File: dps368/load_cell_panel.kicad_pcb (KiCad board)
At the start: 2 copper layers, 50 x 46 mm, 96 parts, among them J1 Conn_01x05_Female, U1 DPS368XTSA1

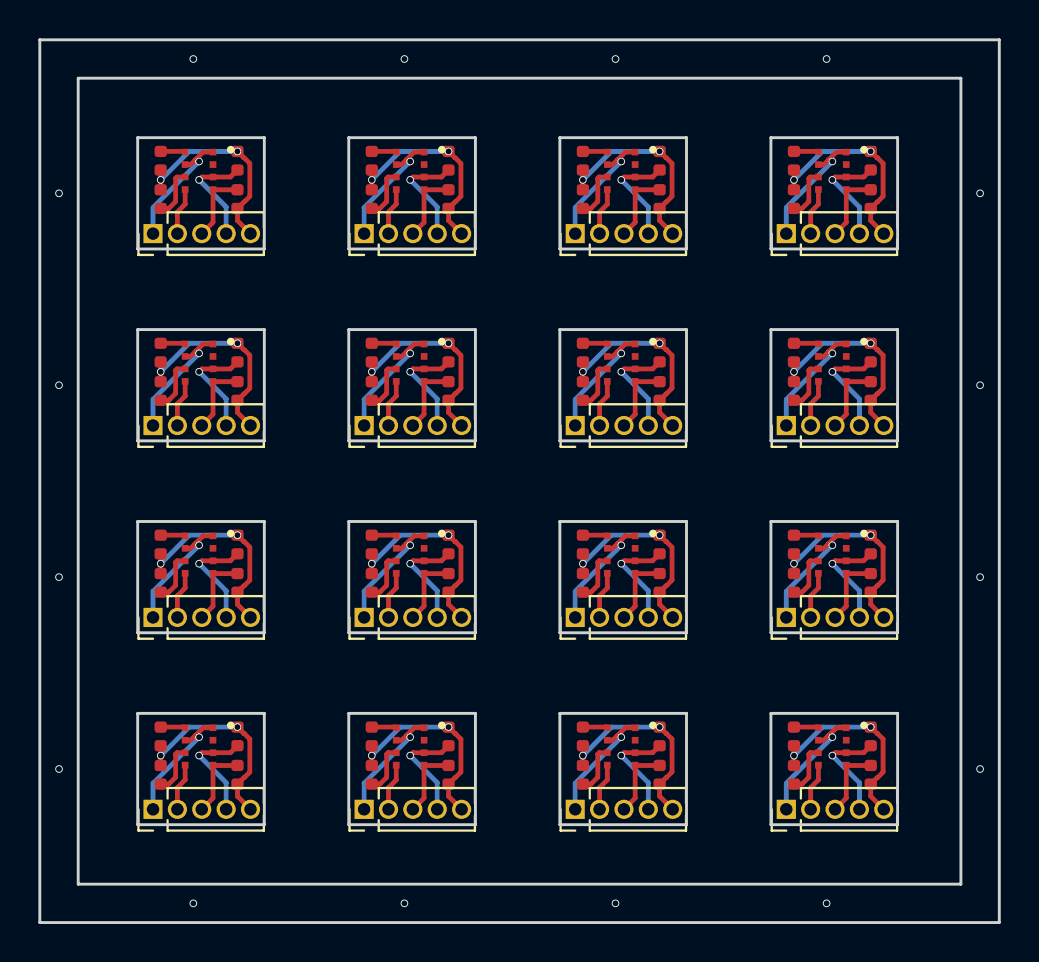
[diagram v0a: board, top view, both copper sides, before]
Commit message: goddamn it
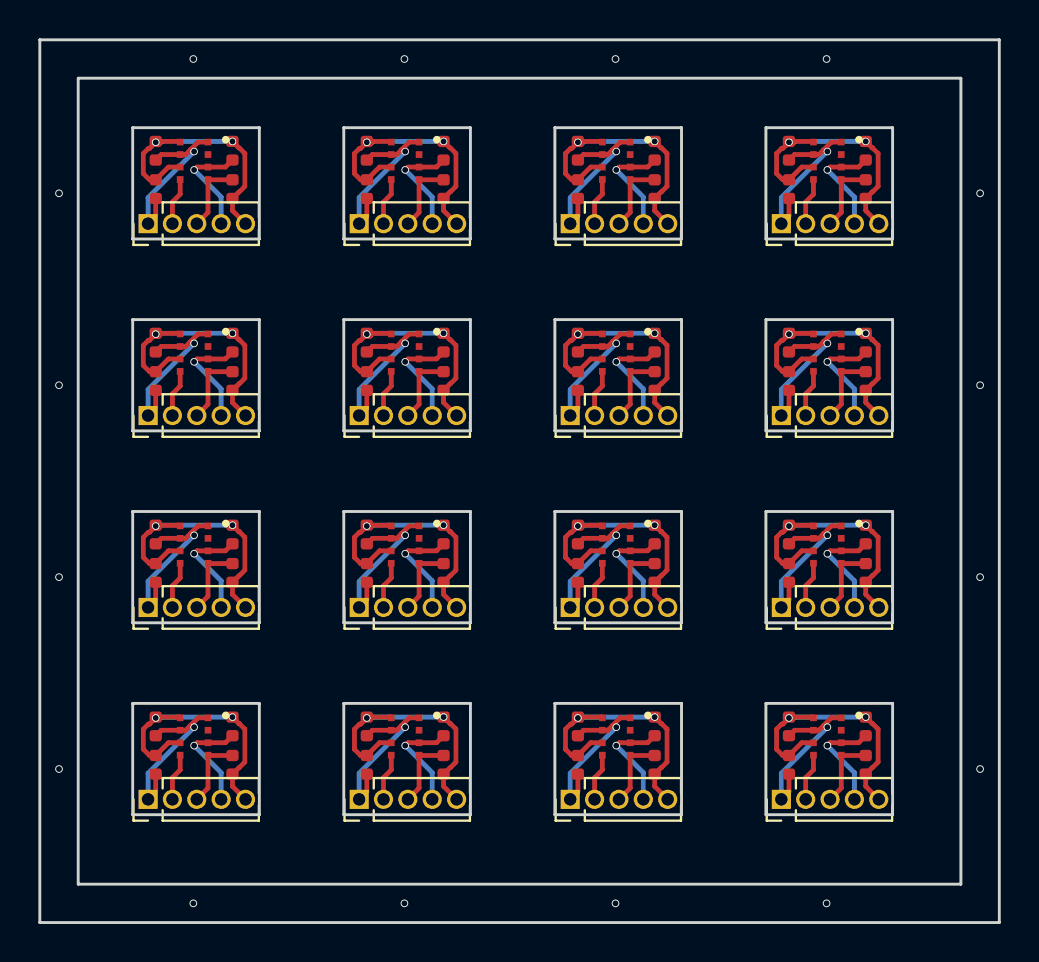
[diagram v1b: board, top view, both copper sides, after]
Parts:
- removed the C1 at (164.3, 101.3)
- removed the C1 at (153.3, 81.3)
- removed the C1 at (142.3, 81.3)
- removed the C1 at (131.3, 81.3)
- removed the C1 at (164.3, 71.3)
- removed the C1 at (153.3, 71.3)
- removed the C1 at (142.3, 71.3)
- removed the C1 at (153.3, 101.3)
- removed the C1 at (142.3, 101.3)
- removed the C1 at (131.3, 101.3)
- removed the C1 at (164.3, 91.3)
- removed the C1 at (153.3, 91.3)
- removed the C1 at (142.3, 91.3)
- removed the C1 at (131.3, 91.3)
- removed the C1 at (164.3, 81.3)
- removed the C2 at (164.3, 103.3)
- removed the C2 at (153.3, 83.3)
- removed the C2 at (142.3, 83.3)
- removed the C2 at (131.3, 83.3)
- removed the C2 at (164.3, 73.3)
- removed the C2 at (153.3, 73.3)
- removed the C2 at (142.3, 73.3)
- removed the C2 at (153.3, 103.3)
- removed the C2 at (142.3, 103.3)
- removed the C2 at (131.3, 103.3)
- removed the C2 at (164.3, 93.3)
- removed the C2 at (153.3, 93.3)
- removed the C2 at (142.3, 93.3)
- removed the C2 at (131.3, 93.3)
- removed the C2 at (164.3, 83.3)
- removed the J1 at (163.9, 105.1)
- removed the J1 at (152.9, 85.1)
- removed the J1 at (141.9, 85.1)
- removed the J1 at (130.9, 85.1)
- removed the J1 at (163.9, 75.1)
- removed the J1 at (152.9, 75.1)
- removed the J1 at (141.9, 75.1)
- removed the J1 at (152.9, 105.1)
- removed the J1 at (141.9, 105.1)
- removed the J1 at (130.9, 105.1)
- removed the J1 at (163.9, 95.1)
- removed the J1 at (152.9, 95.1)
- removed the J1 at (141.9, 95.1)
- removed the J1 at (130.9, 95.1)
- removed the J1 at (163.9, 85.1)
- removed the R1 at (168.3, 103.3)
- removed the R1 at (157.3, 83.3)
- removed the R1 at (146.3, 83.3)
- removed the R1 at (135.3, 83.3)
- removed the R1 at (168.3, 73.3)
- removed the R1 at (157.3, 73.3)
- removed the R1 at (146.3, 73.3)
- removed the R1 at (157.3, 103.3)
- removed the R1 at (146.3, 103.3)
- removed the R1 at (135.3, 103.3)
- removed the R1 at (168.3, 93.3)
- removed the R1 at (157.3, 93.3)
- removed the R1 at (146.3, 93.3)
- removed the R1 at (135.3, 93.3)
- removed the R1 at (168.3, 83.3)
- removed the R2 at (168.3, 101.3)
- removed the R2 at (157.3, 81.3)
- removed the R2 at (146.3, 81.3)
- removed the R2 at (135.3, 81.3)
- removed the R2 at (168.3, 71.3)
- removed the R2 at (157.3, 71.3)
- removed the R2 at (146.3, 71.3)
- removed the R2 at (157.3, 101.3)
- removed the R2 at (146.3, 101.3)
- removed the R2 at (135.3, 101.3)
- removed the R2 at (168.3, 91.3)
- removed the R2 at (157.3, 91.3)
- removed the R2 at (146.3, 91.3)
- removed the R2 at (135.3, 91.3)
- removed the R2 at (168.3, 81.3)
- removed the U1 at (166.3, 101.8)
- removed the U1 at (155.3, 81.8)
- removed the U1 at (144.3, 81.8)
- removed the U1 at (133.3, 81.8)
- removed the U1 at (166.3, 71.8)
- removed the U1 at (155.3, 71.8)
- removed the U1 at (144.3, 71.8)
- removed the U1 at (155.3, 101.8)
- removed the U1 at (144.3, 101.8)
- removed the U1 at (133.3, 101.8)
- removed the U1 at (166.3, 91.8)
- removed the U1 at (155.3, 91.8)
- removed the U1 at (144.3, 91.8)
- removed the U1 at (133.3, 91.8)
- removed the U1 at (166.3, 81.8)
- added C1: 100n, Capacitor_SMD:C_0402_1005Metric, F.Cu at (164.0, 100.8)
- added C1: 100n, Capacitor_SMD:C_0402_1005Metric, F.Cu at (153.0, 80.8)
- added C1: 100n, Capacitor_SMD:C_0402_1005Metric, F.Cu at (142.0, 80.8)
- added C1: 100n, Capacitor_SMD:C_0402_1005Metric, F.Cu at (131.0, 80.8)
- added C1: 100n, Capacitor_SMD:C_0402_1005Metric, F.Cu at (164.0, 70.8)
- added C1: 100n, Capacitor_SMD:C_0402_1005Metric, F.Cu at (153.0, 70.8)
- added C1: 100n, Capacitor_SMD:C_0402_1005Metric, F.Cu at (142.0, 70.8)
- added C1: 100n, Capacitor_SMD:C_0402_1005Metric, F.Cu at (153.0, 100.8)
- added C1: 100n, Capacitor_SMD:C_0402_1005Metric, F.Cu at (142.0, 100.8)
- added C1: 100n, Capacitor_SMD:C_0402_1005Metric, F.Cu at (131.0, 100.8)
- added C1: 100n, Capacitor_SMD:C_0402_1005Metric, F.Cu at (164.0, 90.8)
- added C1: 100n, Capacitor_SMD:C_0402_1005Metric, F.Cu at (153.0, 90.8)
- added C1: 100n, Capacitor_SMD:C_0402_1005Metric, F.Cu at (142.0, 90.8)
- added C1: 100n, Capacitor_SMD:C_0402_1005Metric, F.Cu at (131.0, 90.8)
- added C1: 100n, Capacitor_SMD:C_0402_1005Metric, F.Cu at (164.0, 80.8)
- added C2: 100n, Capacitor_SMD:C_0402_1005Metric, F.Cu at (164.0, 102.8)
- added C2: 100n, Capacitor_SMD:C_0402_1005Metric, F.Cu at (153.0, 82.8)
- added C2: 100n, Capacitor_SMD:C_0402_1005Metric, F.Cu at (142.0, 82.8)
- added C2: 100n, Capacitor_SMD:C_0402_1005Metric, F.Cu at (131.0, 82.8)
- added C2: 100n, Capacitor_SMD:C_0402_1005Metric, F.Cu at (164.0, 72.8)
- added C2: 100n, Capacitor_SMD:C_0402_1005Metric, F.Cu at (153.0, 72.8)
- added C2: 100n, Capacitor_SMD:C_0402_1005Metric, F.Cu at (142.0, 72.8)
- added C2: 100n, Capacitor_SMD:C_0402_1005Metric, F.Cu at (153.0, 102.8)
- added C2: 100n, Capacitor_SMD:C_0402_1005Metric, F.Cu at (142.0, 102.8)
- added C2: 100n, Capacitor_SMD:C_0402_1005Metric, F.Cu at (131.0, 102.8)
- added C2: 100n, Capacitor_SMD:C_0402_1005Metric, F.Cu at (164.0, 92.8)
- added C2: 100n, Capacitor_SMD:C_0402_1005Metric, F.Cu at (153.0, 92.8)
- added C2: 100n, Capacitor_SMD:C_0402_1005Metric, F.Cu at (142.0, 92.8)
- added C2: 100n, Capacitor_SMD:C_0402_1005Metric, F.Cu at (131.0, 92.8)
- added C2: 100n, Capacitor_SMD:C_0402_1005Metric, F.Cu at (164.0, 82.8)
- added J1: Conn_01x05_Female, Connector_PinHeader_1.27mm:PinHeader_1x05_P1.27mm_Vertical, F.Cu at (163.6, 104.6)
- added J1: Conn_01x05_Female, Connector_PinHeader_1.27mm:PinHeader_1x05_P1.27mm_Vertical, F.Cu at (152.6, 84.6)
- added J1: Conn_01x05_Female, Connector_PinHeader_1.27mm:PinHeader_1x05_P1.27mm_Vertical, F.Cu at (141.6, 84.6)
- added J1: Conn_01x05_Female, Connector_PinHeader_1.27mm:PinHeader_1x05_P1.27mm_Vertical, F.Cu at (130.6, 84.6)
- added J1: Conn_01x05_Female, Connector_PinHeader_1.27mm:PinHeader_1x05_P1.27mm_Vertical, F.Cu at (163.6, 74.6)
- added J1: Conn_01x05_Female, Connector_PinHeader_1.27mm:PinHeader_1x05_P1.27mm_Vertical, F.Cu at (152.6, 74.6)
- added J1: Conn_01x05_Female, Connector_PinHeader_1.27mm:PinHeader_1x05_P1.27mm_Vertical, F.Cu at (141.6, 74.6)
- added J1: Conn_01x05_Female, Connector_PinHeader_1.27mm:PinHeader_1x05_P1.27mm_Vertical, F.Cu at (152.6, 104.6)
- added J1: Conn_01x05_Female, Connector_PinHeader_1.27mm:PinHeader_1x05_P1.27mm_Vertical, F.Cu at (141.6, 104.6)
- added J1: Conn_01x05_Female, Connector_PinHeader_1.27mm:PinHeader_1x05_P1.27mm_Vertical, F.Cu at (130.6, 104.6)
- added J1: Conn_01x05_Female, Connector_PinHeader_1.27mm:PinHeader_1x05_P1.27mm_Vertical, F.Cu at (163.6, 94.6)
- added J1: Conn_01x05_Female, Connector_PinHeader_1.27mm:PinHeader_1x05_P1.27mm_Vertical, F.Cu at (152.6, 94.6)
- added J1: Conn_01x05_Female, Connector_PinHeader_1.27mm:PinHeader_1x05_P1.27mm_Vertical, F.Cu at (141.6, 94.6)
- added J1: Conn_01x05_Female, Connector_PinHeader_1.27mm:PinHeader_1x05_P1.27mm_Vertical, F.Cu at (130.6, 94.6)
- added J1: Conn_01x05_Female, Connector_PinHeader_1.27mm:PinHeader_1x05_P1.27mm_Vertical, F.Cu at (163.6, 84.6)
- added R1: 10k, Resistor_SMD:R_0402_1005Metric, F.Cu at (168.0, 102.8)
- added R1: 10k, Resistor_SMD:R_0402_1005Metric, F.Cu at (157.0, 82.8)
- added R1: 10k, Resistor_SMD:R_0402_1005Metric, F.Cu at (146.0, 82.8)
- added R1: 10k, Resistor_SMD:R_0402_1005Metric, F.Cu at (135.0, 82.8)
- added R1: 10k, Resistor_SMD:R_0402_1005Metric, F.Cu at (168.0, 72.8)
- added R1: 10k, Resistor_SMD:R_0402_1005Metric, F.Cu at (157.0, 72.8)
- added R1: 10k, Resistor_SMD:R_0402_1005Metric, F.Cu at (146.0, 72.8)
- added R1: 10k, Resistor_SMD:R_0402_1005Metric, F.Cu at (157.0, 102.8)
- added R1: 10k, Resistor_SMD:R_0402_1005Metric, F.Cu at (146.0, 102.8)
- added R1: 10k, Resistor_SMD:R_0402_1005Metric, F.Cu at (135.0, 102.8)
- added R1: 10k, Resistor_SMD:R_0402_1005Metric, F.Cu at (168.0, 92.8)
- added R1: 10k, Resistor_SMD:R_0402_1005Metric, F.Cu at (157.0, 92.8)
- added R1: 10k, Resistor_SMD:R_0402_1005Metric, F.Cu at (146.0, 92.8)
- added R1: 10k, Resistor_SMD:R_0402_1005Metric, F.Cu at (135.0, 92.8)
- added R1: 10k, Resistor_SMD:R_0402_1005Metric, F.Cu at (168.0, 82.8)
- added R2: 10k, Resistor_SMD:R_0402_1005Metric, F.Cu at (168.0, 100.8)
- added R2: 10k, Resistor_SMD:R_0402_1005Metric, F.Cu at (157.0, 80.8)
- added R2: 10k, Resistor_SMD:R_0402_1005Metric, F.Cu at (146.0, 80.8)
- added R2: 10k, Resistor_SMD:R_0402_1005Metric, F.Cu at (135.0, 80.8)
- added R2: 10k, Resistor_SMD:R_0402_1005Metric, F.Cu at (168.0, 70.8)
- added R2: 10k, Resistor_SMD:R_0402_1005Metric, F.Cu at (157.0, 70.8)
- added R2: 10k, Resistor_SMD:R_0402_1005Metric, F.Cu at (146.0, 70.8)
- added R2: 10k, Resistor_SMD:R_0402_1005Metric, F.Cu at (157.0, 100.8)
- added R2: 10k, Resistor_SMD:R_0402_1005Metric, F.Cu at (146.0, 100.8)
- added R2: 10k, Resistor_SMD:R_0402_1005Metric, F.Cu at (135.0, 100.8)
- added R2: 10k, Resistor_SMD:R_0402_1005Metric, F.Cu at (168.0, 90.8)
- added R2: 10k, Resistor_SMD:R_0402_1005Metric, F.Cu at (157.0, 90.8)
- added R2: 10k, Resistor_SMD:R_0402_1005Metric, F.Cu at (146.0, 90.8)
- added R2: 10k, Resistor_SMD:R_0402_1005Metric, F.Cu at (135.0, 90.8)
- added R2: 10k, Resistor_SMD:R_0402_1005Metric, F.Cu at (168.0, 80.8)
- added U1: DPS368XTSA1, custom_lib:XDCR_DPS368XTSA1, F.Cu at (166.0, 101.3)
- added U1: DPS368XTSA1, custom_lib:XDCR_DPS368XTSA1, F.Cu at (155.0, 81.3)
- added U1: DPS368XTSA1, custom_lib:XDCR_DPS368XTSA1, F.Cu at (144.0, 81.3)
- added U1: DPS368XTSA1, custom_lib:XDCR_DPS368XTSA1, F.Cu at (133.0, 81.3)
- added U1: DPS368XTSA1, custom_lib:XDCR_DPS368XTSA1, F.Cu at (166.0, 71.3)
- added U1: DPS368XTSA1, custom_lib:XDCR_DPS368XTSA1, F.Cu at (155.0, 71.3)
- added U1: DPS368XTSA1, custom_lib:XDCR_DPS368XTSA1, F.Cu at (144.0, 71.3)
- added U1: DPS368XTSA1, custom_lib:XDCR_DPS368XTSA1, F.Cu at (155.0, 101.3)
- added U1: DPS368XTSA1, custom_lib:XDCR_DPS368XTSA1, F.Cu at (144.0, 101.3)
- added U1: DPS368XTSA1, custom_lib:XDCR_DPS368XTSA1, F.Cu at (133.0, 101.3)
- added U1: DPS368XTSA1, custom_lib:XDCR_DPS368XTSA1, F.Cu at (166.0, 91.3)
- added U1: DPS368XTSA1, custom_lib:XDCR_DPS368XTSA1, F.Cu at (155.0, 91.3)
- added U1: DPS368XTSA1, custom_lib:XDCR_DPS368XTSA1, F.Cu at (144.0, 91.3)
- added U1: DPS368XTSA1, custom_lib:XDCR_DPS368XTSA1, F.Cu at (133.0, 91.3)
- added U1: DPS368XTSA1, custom_lib:XDCR_DPS368XTSA1, F.Cu at (166.0, 81.3)
- moved C1 0.58 mm to (131.0, 70.8)
- moved C2 0.58 mm to (131.0, 72.8)
- moved J1 0.58 mm to (130.6, 74.6)
- moved R1 0.58 mm to (135.0, 72.8)
- moved R2 0.58 mm to (135.0, 70.8)
- moved U1 0.58 mm to (133.0, 71.3)
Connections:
- C1 pad 1: +3V3 -> GND
- C1 pad 2: Net-(C1-Pad2) -> +3V3
- C2 pad 1: Net-(C2-Pad1) -> GND
- U1 pad 6: Net-(C2-Pad1) -> +3V3
- U1 pad 8: Net-(C1-Pad2) -> +3V3
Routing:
- net +3V3: track 172.3 -> 235.8 mm
- net GND: track 107.3 -> 153.3 mm
- net Net-(C2-Pad1): track 42.5 -> 0.00 mm
- net Net-(C1-Pad2): track 20.6 -> 0.00 mm
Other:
- outline, holes or cut-outs redrawn
